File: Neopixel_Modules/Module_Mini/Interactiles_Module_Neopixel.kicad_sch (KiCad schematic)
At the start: 29 parts, among them J1 PINHD_1x2_Male, J2 PINHD_1x2_Female, J4 PINHD_1x2_Female, U1 MCP23017_ML

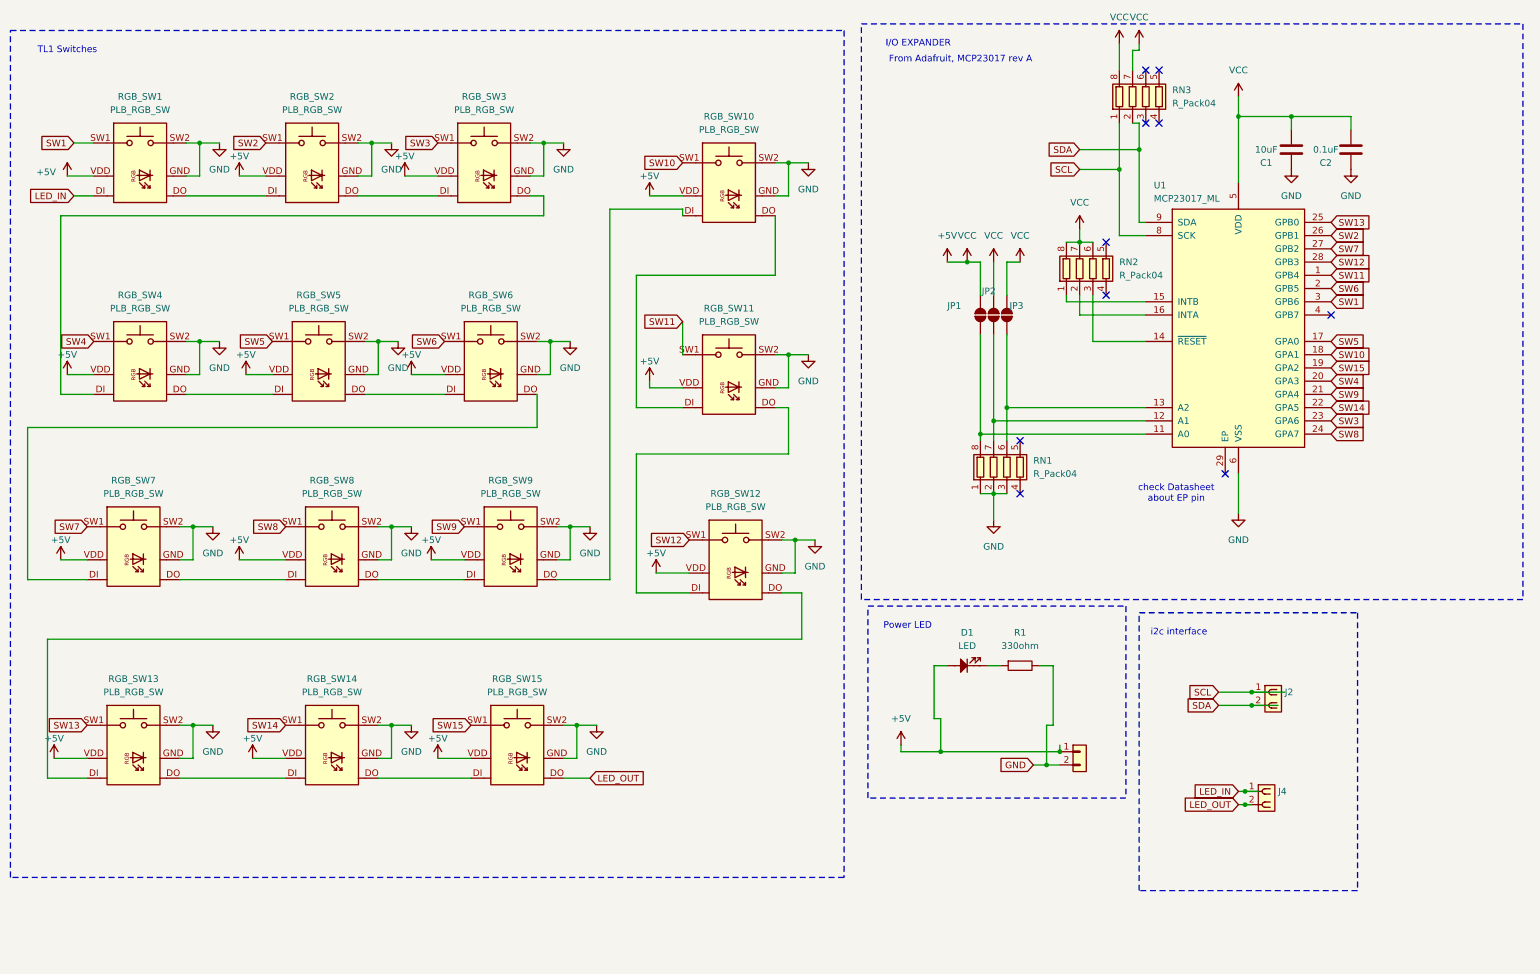
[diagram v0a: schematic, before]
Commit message: fixed for pcb production
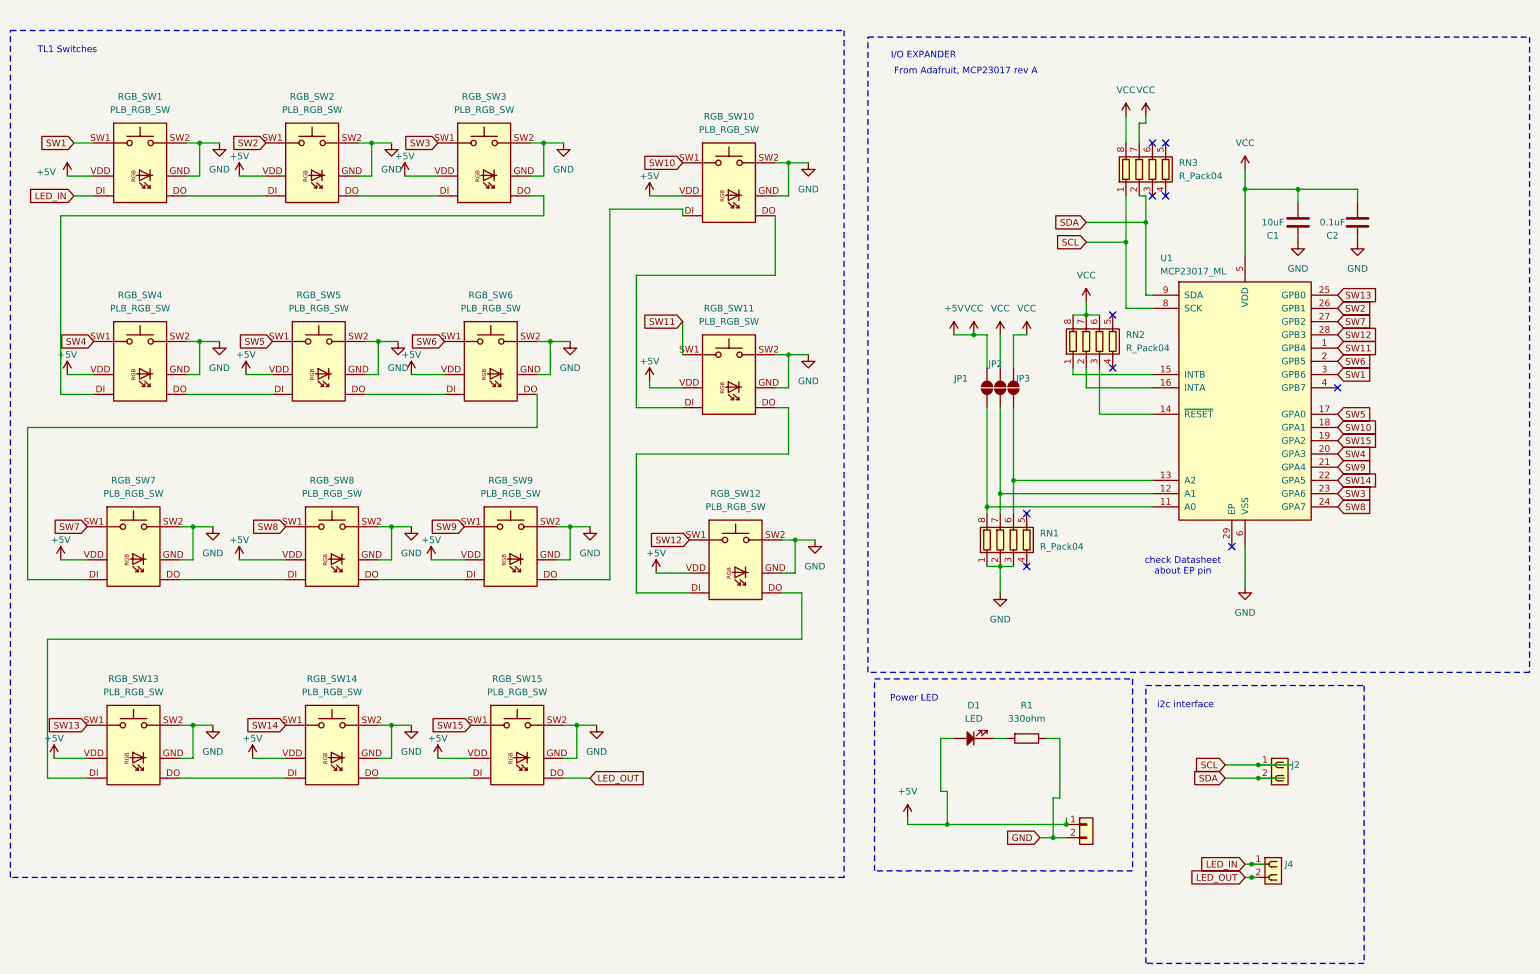
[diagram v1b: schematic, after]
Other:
- moved on the sheet: C1, C2, D1, J2, J4, JP1, JP2, JP3, R1, RN1, RN2, RN3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
